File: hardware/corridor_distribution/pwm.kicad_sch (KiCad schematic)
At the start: 9 parts, among them U2 PCA9635, U3 PCA9685PW

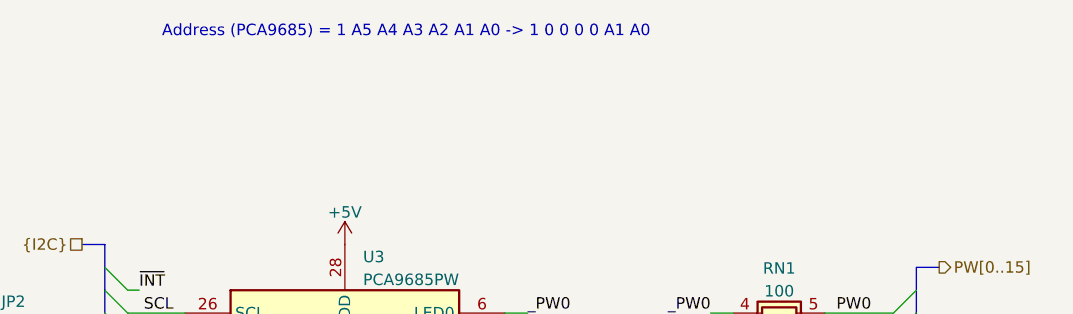
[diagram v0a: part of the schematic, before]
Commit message: Night Light firmware
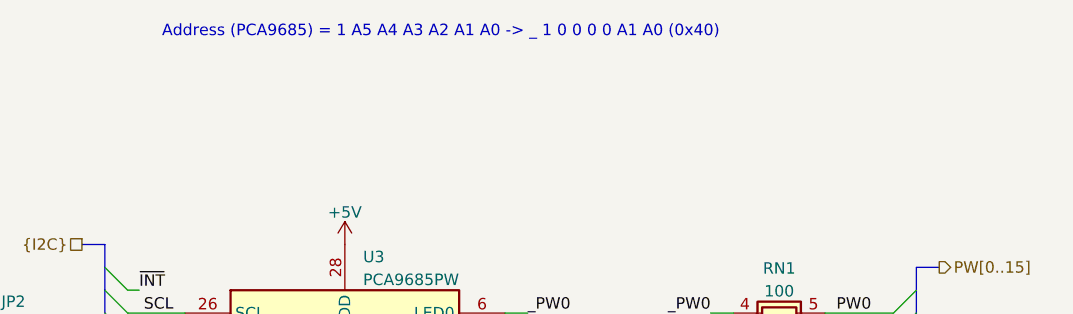
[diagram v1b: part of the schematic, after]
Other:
- note added: "Address (PCA9685) = 1 A5 A4 A3 A2 A1 A0 -> _ 1 0 0 0 0 A1 A0 (0x40)"
- note removed: "Address (PCA9685) = 1 A5 A4 A3 A2 A1 A0 -> 1 0 0 0 0 A1 A0"
